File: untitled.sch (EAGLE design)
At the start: 116 parts, among them IC4 MCP23017SS, K2 351, Q1 S9013, U49 PC817X2NIP0F

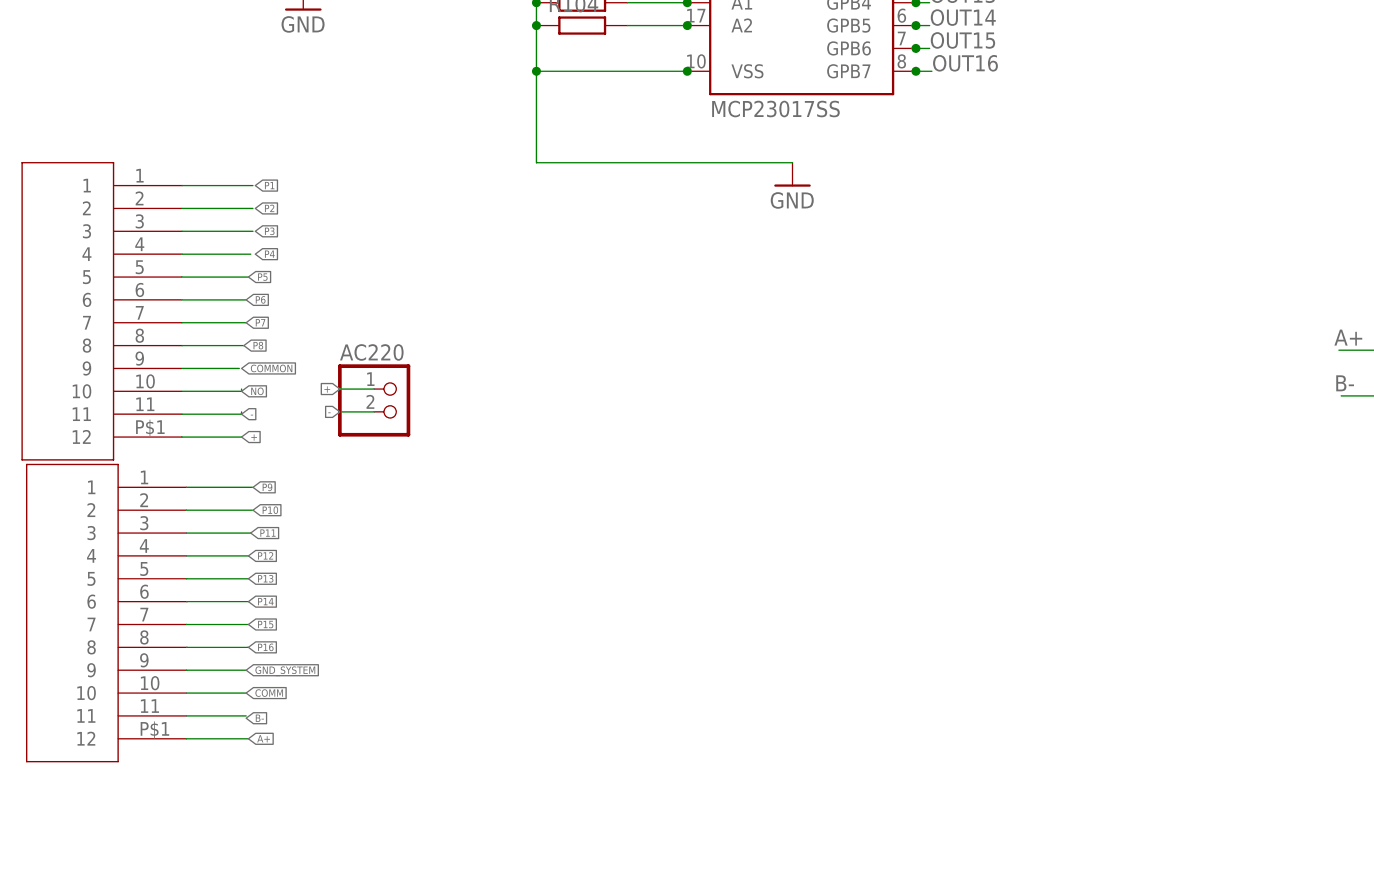
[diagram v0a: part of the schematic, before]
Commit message: revisi PCB
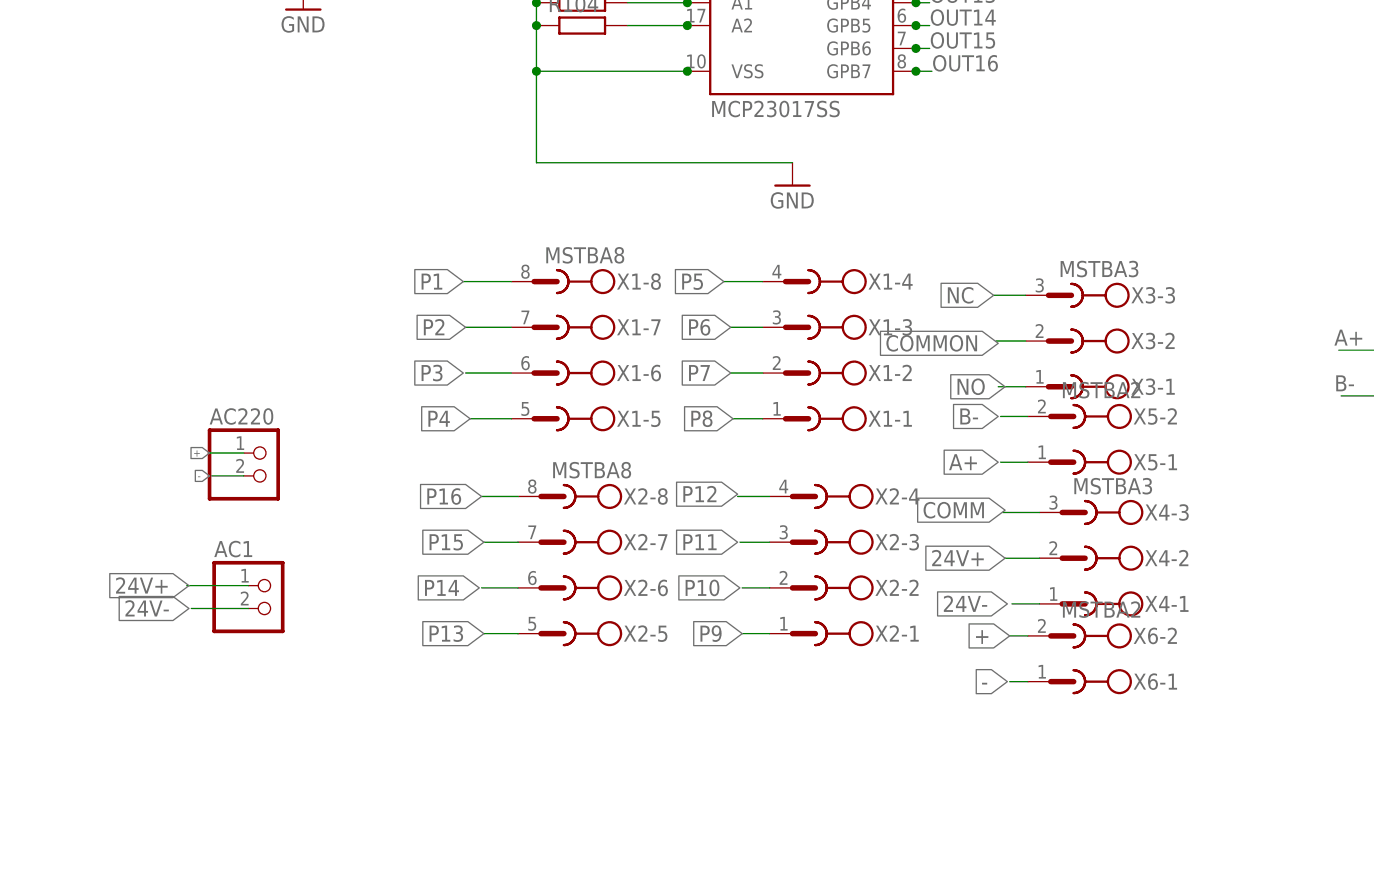
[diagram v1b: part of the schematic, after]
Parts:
- removed TERMINAL-BLOCK10P1, TERMINAL-BLOCK10P2: (no value), terminal-blok10p:TERMINAL-BLOCK10P
- added AC1: (no value), pinhead:PINHD-1X2
- added X1, X2: MSTBA8, con-phoenix-508:MSTBA8
- added X3, X4: MSTBA3, con-phoenix-508:MSTBA3
- added X5, X6: MSTBA2, con-phoenix-508:MSTBA2
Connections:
- removed net GND_SYSTEM: TERMINAL-BLOCK10P2.9
- new net 24V+: AC1.1, X4-2.1
- new net 24V-: AC1.2, X4-1.1
- net +: now also X6-2.1; no longer TERMINAL-BLOCK10P1.12
- net -: now also X6-1.1; no longer TERMINAL-BLOCK10P1.11
- net A+: now also X5-1.1; no longer TERMINAL-BLOCK10P2.12
- net B-: now also X5-2.1; no longer TERMINAL-BLOCK10P2.11
- net COMM: now also X4-3.1; no longer TERMINAL-BLOCK10P2.10
- net COMMON: now also X3-2.1; no longer TERMINAL-BLOCK10P1.9
- net NC: now also X3-3.1
- net NO: now also X3-1.1; no longer TERMINAL-BLOCK10P1.10
- net P1: now also X1-8.1; no longer TERMINAL-BLOCK10P1.1
- net P10: now also X2-2.1; no longer TERMINAL-BLOCK10P2.2
- net P11: now also X2-3.1; no longer TERMINAL-BLOCK10P2.3
- net P12: now also X2-4.1; no longer TERMINAL-BLOCK10P2.4
- net P13: now also X2-5.1; no longer TERMINAL-BLOCK10P2.5
- net P14: now also X2-6.1; no longer TERMINAL-BLOCK10P2.6
- net P15: now also X2-7.1; no longer TERMINAL-BLOCK10P2.7
- net P16: now also X2-8.1; no longer TERMINAL-BLOCK10P2.8
- net P2: now also X1-7.1; no longer TERMINAL-BLOCK10P1.2
- net P3: now also X1-6.1; no longer TERMINAL-BLOCK10P1.3
- net P4: now also X1-5.1; no longer TERMINAL-BLOCK10P1.4
- net P5: now also X1-4.1; no longer TERMINAL-BLOCK10P1.5
- net P6: now also X1-3.1; no longer TERMINAL-BLOCK10P1.6
- net P7: now also X1-2.1; no longer TERMINAL-BLOCK10P1.7
- net P8: now also X1-1.1; no longer TERMINAL-BLOCK10P1.8
- net P9: now also X2-1.1; no longer TERMINAL-BLOCK10P2.1
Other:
- moved on the sheet: AC220
